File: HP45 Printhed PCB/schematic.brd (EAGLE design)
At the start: 35 x 62 mm, 40 parts, among them P1 0930, P2 0930, P3 0930, P4 0930

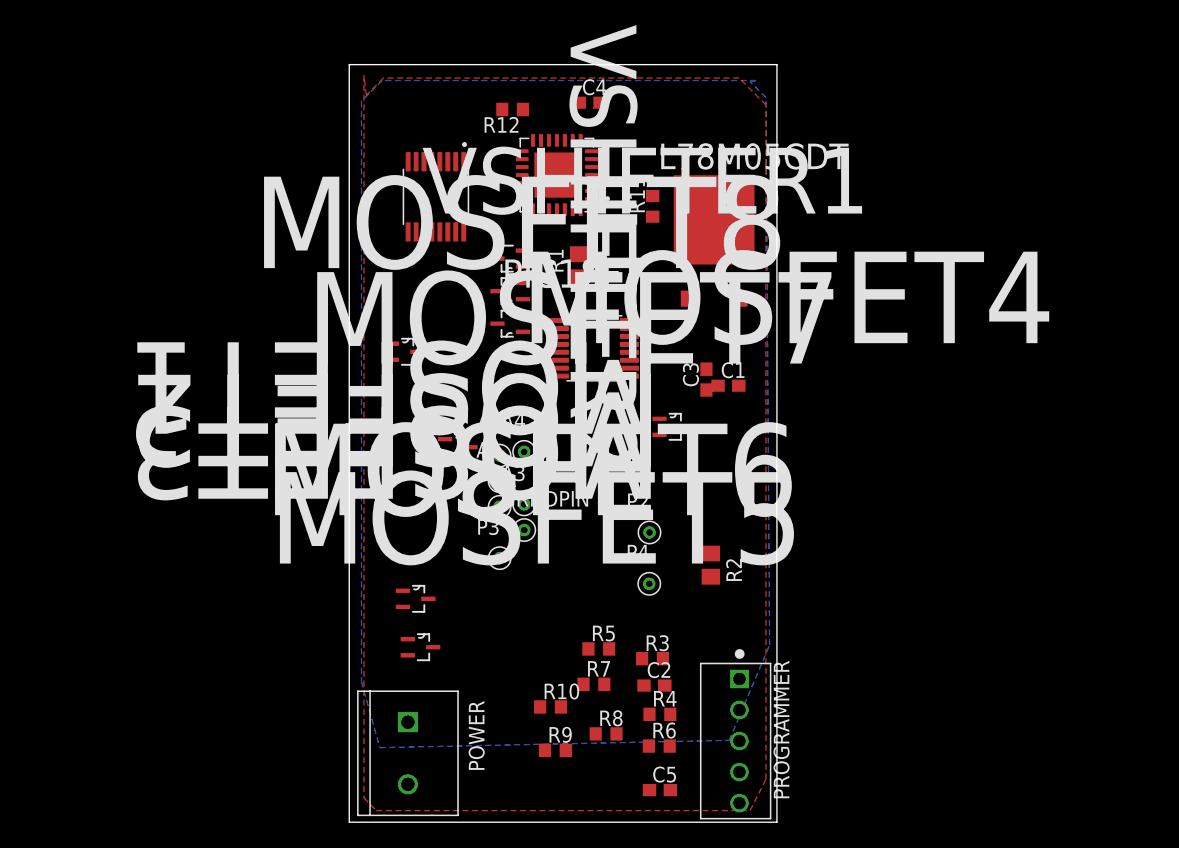
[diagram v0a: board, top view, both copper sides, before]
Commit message: PCB
Done
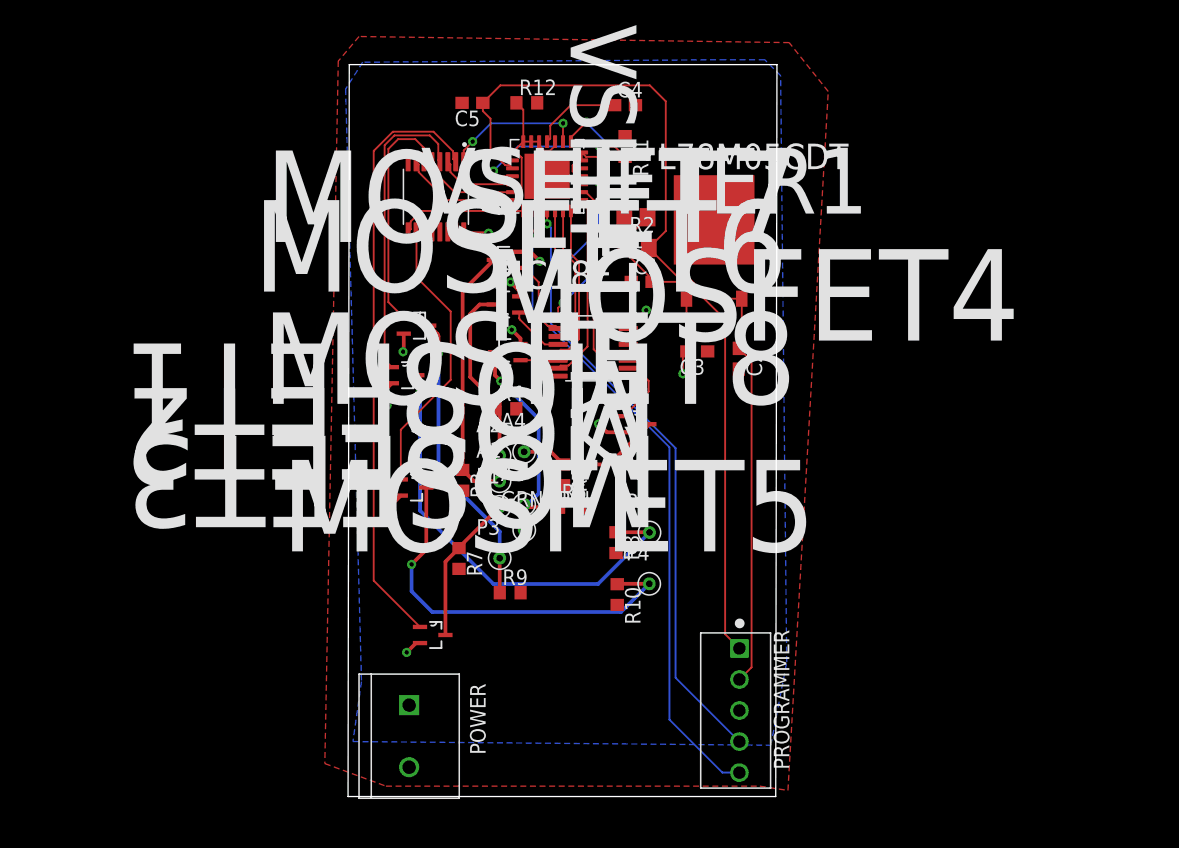
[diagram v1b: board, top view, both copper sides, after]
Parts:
- moved C5 58.3 mm to (10.1, 58.9), turned to 180 degrees
- moved R4 28.0 mm to (12.8, 33.8)
- moved C2 27.6 mm to (31.9, 37.9), turned to 270 degrees
- moved R2 26.6 mm to (23.6, 47.0), turned to 0 degrees
- moved R6 23.5 mm to (17.5, 28.4), turned to 270 degrees
- moved R3 21.3 mm to (9.28, 28.0), turned to 270 degrees
- moved MOSFET6 18.3 mm to (4.53, 36.6)
- moved R8 15.7 mm to (21.8, 22.9), turned to 270 degrees
- moved R7 15.1 mm to (8.98, 21.6), turned to 270 degrees
- moved R9 13.4 mm to (13.2, 18.8)
- moved R5 11.8 mm to (18.0, 25.8)
- moved MOSFET8 11.1 mm to (5.26, 27.4)
- moved C1 11.1 mm to (23.9, 44.2)
- moved R10 10.7 mm to (21.9, 18.6), turned to 270 degrees
- moved MOSFET7 10.5 mm to (5.50, 40.6)
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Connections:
- net PICKIT_VDD: now also L78M05CDT.3
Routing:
- net PICKIT_VDD: track 0.00 -> 76.8 mm
- net PIC_PGC: track 0.00 -> 54.3 mm, vias 0 -> 1
- net PIC_PGD: track 0.00 -> 49.9 mm, vias 0 -> 1
- net HEAD_P1: track 0.00 -> 49.3 mm
- net PICKIT_MCLR: track 0.00 -> 41.7 mm
- net N$9: track 0.00 -> 36.9 mm, vias 0 -> 1
- net N$11: track 0.00 -> 32.7 mm, vias 0 -> 1
- net HEAD_P2: track 0.00 -> 24.9 mm
- net N$10: track 0.00 -> 24.3 mm, vias 0 -> 1
- net +12V: track 0.00 -> 24.1 mm, vias 0 -> 11
- net HEAD_P4: track 0.00 -> 23.1 mm
- net N$2: track 0.00 -> 21.6 mm
- net N$3: track 0.00 -> 21.0 mm, vias 0 -> 2
- net SHIFTER_VCC_A: track 0.00 -> 20.7 mm, vias 0 -> 2
- net HEAD_P3: track 0.00 -> 19.0 mm
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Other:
- board size 35 x 62 mm -> 35.1 x 59.9 mm
